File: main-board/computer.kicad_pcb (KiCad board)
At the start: 2 copper layers, 141 x 76.8 mm, 26 parts, among them J1 Conn_02x20_Odd_Even, J2 Conn_02x20_Odd_Even, J3 PORT A, J4 PORT B, J5 SERIAL, SW1 RESET, U1 W65C02S, U11 DS1813, U2 AS6C62256-55, U3 SST39SF010, U4 W65C22N, U5 W65C51N, U6 74HC00, U7 74HC30, U8 74HC138, X1 1.8432MHz

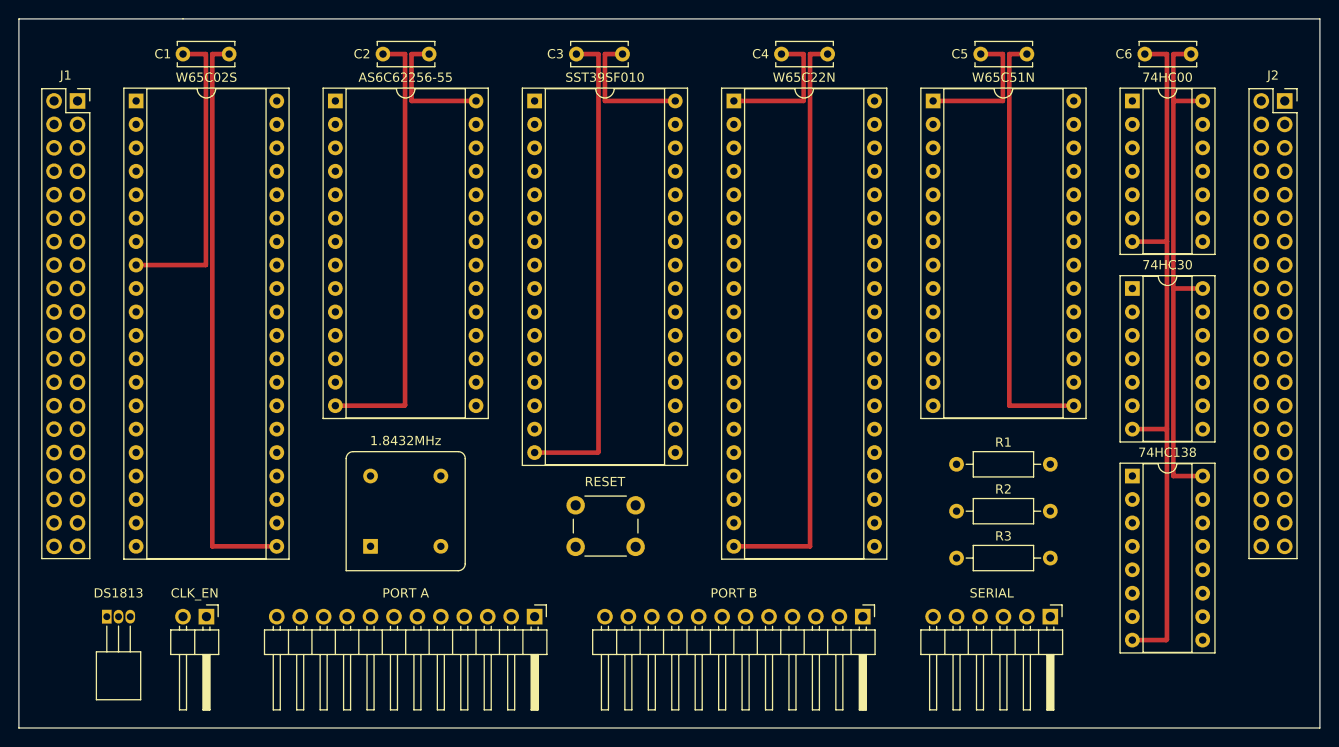
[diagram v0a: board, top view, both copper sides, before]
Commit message: More on layouts
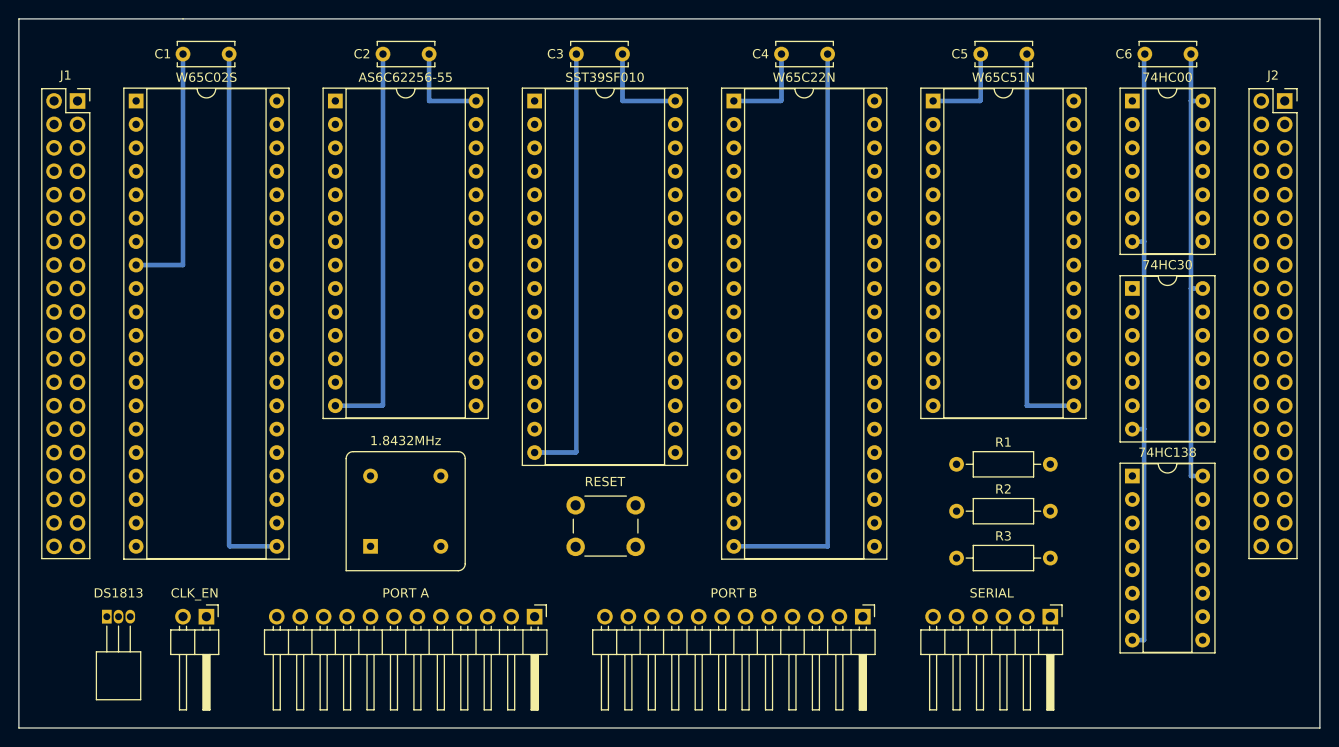
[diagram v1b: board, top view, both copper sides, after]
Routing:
- net GND: track 269.8 -> 237.1 mm
- net +5V: track 229.1 -> 205.1 mm

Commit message: Revert "More on layouts"
This reverts commit 3fc7c4d1a32f245eaa0a26aebed00be081417dbd.
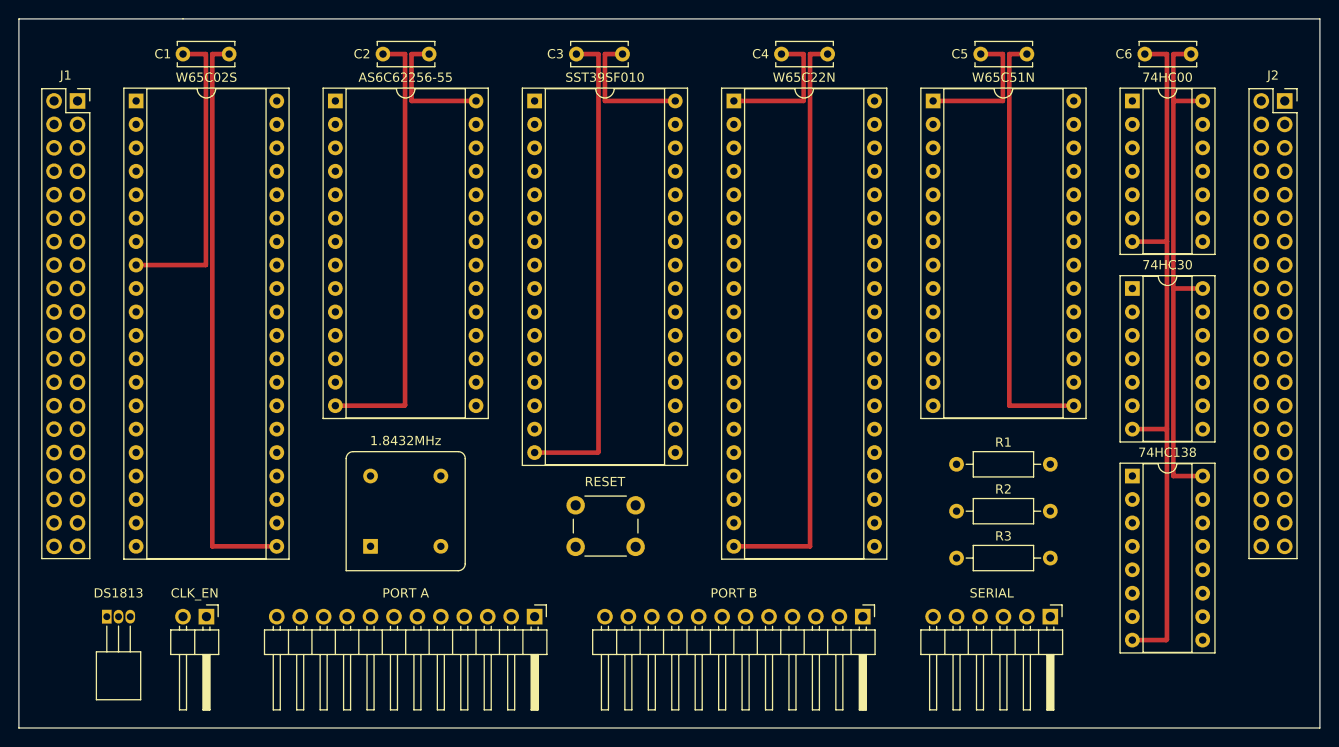
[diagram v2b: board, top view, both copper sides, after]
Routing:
- net GND: track 237.1 -> 269.8 mm
- net +5V: track 205.1 -> 229.1 mm
